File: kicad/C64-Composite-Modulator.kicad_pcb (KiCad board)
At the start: 2 copper layers, 63.5 x 60 mm, 56 parts, among them J1 Conn_01x04_Male, J2 Conn_01x04_Male, J3 Conn_01x04_Male, J4 Conn_01x04_Male, Q1 BC847B, Q2 BC847B, U1 78L05

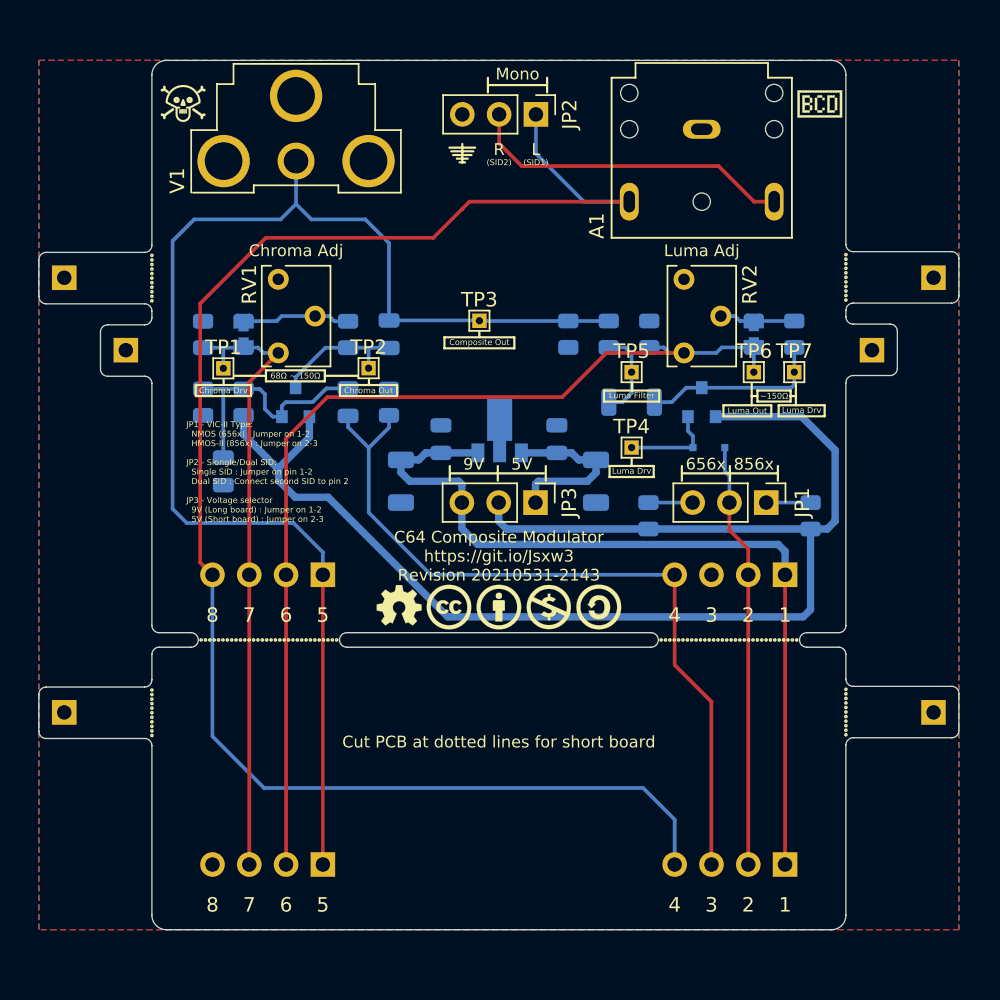
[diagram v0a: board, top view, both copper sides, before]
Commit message: Revision 20220130-1040
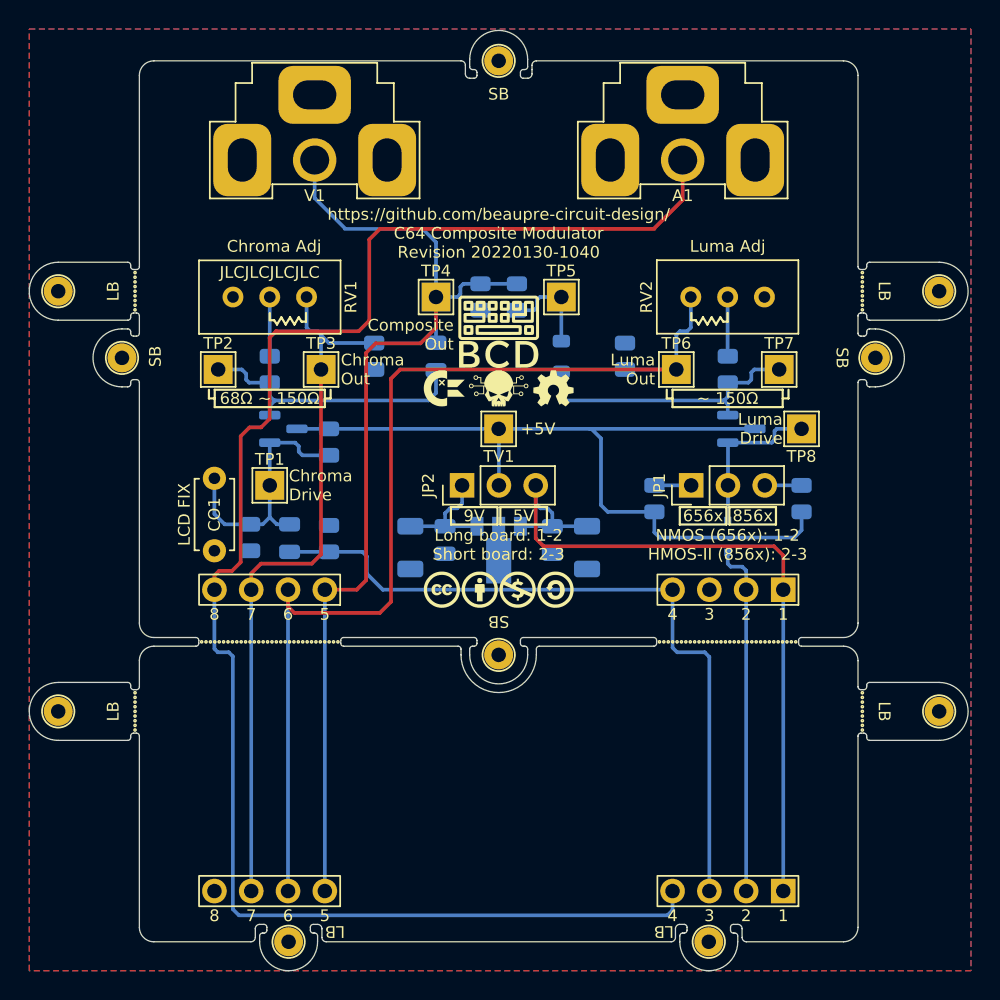
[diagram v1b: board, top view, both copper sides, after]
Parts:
- removed B1: RV1 Bypass, C64 Composite Modulator:J_0805_2012Metric
- removed B2: RV2 Bypass, C64 Composite Modulator:J_0805_2012Metric
- removed BCD1: BCD(DOT), BCD:BCD_LOGO_DOT-xxxsmall
- removed BY1: CC-BY, BCD:CC-BY-xxxsmall
- removed CC1: CC, BCD:CC-Logo-xxxsmall
- removed Danger1: Danger, BCD:Danger-xxxsmall
- removed J1, J2, J3, J4: Conn_01x04_Male, C64 Composite Modulator:mill-max-800-10-004-10-001000
- removed JP3: Jumper_3_Open, Connector_PinHeader_2.54mm:PinHeader_1x03_P2.54mm_Vertical
- removed LB1, LB2, LB3, LB4, SB1, SB2: Conn_01x01_Male, C64 Composite Modulator:mill-max-800-10-001-10-001000
- removed NC1: CC-NC, BCD:CC-NC-xxxsmall
- removed OSHW1: OSHW, BCD:OSHW-xxxsmall
- removed SA1: CC-SA, BCD:CC-SA-xxxsmall
- added CLB1: Modulator_Board_To_Long_Board, C64 Composite Modulator:Modulator to Long-Board support, F.Cu at (140.8, 105.4)
- added CSB1: Modulator_Board_To_Short_Board, C64 Composite Modulator:Modulator to Short-Board support, F.Cu at (140.8, 104.9)
- added G1: BCD_Logo, BeaupreCircuitDesign:BCD_Logo_5mm, F.Cu at (140.8, 93.7)
- added G2: ChickenLips, BeaupreCircuitDesign:ChickenLips_2.5mm, F.Cu at (137.0, 97.6)
- added G3: OpenSource_Hardware, BeaupreCircuitDesign:Open_Source_Hardware_2.5mm, F.Cu at (144.6, 97.6)
- added G4: Skull, BeaupreCircuitDesign:Skull_2.5mm, F.Cu at (140.8, 97.6)
- added G5: CreativeCommons, Creative_Common:CreativeCommons_2.5mm, F.Cu at (136.9, 111.5)
- added G6: CreativeCommons_Attribution, Creative_Common:CreativeCommons_Attribution_2.5mm, F.Cu at (139.5, 111.5)
- added G7: CreativeCommons_NonCommercial, Creative_Common:CreativeCommons_NonCommercial_2.5mm, F.Cu at (142.1, 111.5)
- added G8: CreativeCommons_ShareAlike, Creative_Common:CreativeCommons_ShareAlike_2.5mm, F.Cu at (144.7, 111.5)
- added TP8: TestPoint, TestPoint:TestPoint_THTPad_2.0x2.0mm_Drill1.0mm, F.Cu at (161.7, 100.4)
- added TV1: TestPoint, TestPoint:TestPoint_THTPad_2.0x2.0mm_Drill1.0mm, F.Cu at (140.8, 100.4)
- A1: value SJ1-3523N -> Conn_Coaxial; footprint C64 Composite Modulator:CUI_SJ1-3523N -> CUI_Devices:RCJ-013
- CO1: renamed from C7; footprint Capacitor_SMD:C_0805_2012Metric -> Capacitor_THT:C_Disc_D4.7mm_W2.5mm_P5.00mm; moved to F.Cu
- D1: value 1N4148 -> 1N4148WS
- L1: footprint Inductor_SMD:L_1206_3216Metric -> Inductor_SMD:L_0805_2012Metric
- Q1, Q2: value BC847B -> BC847C
- R1, R7: value 1K -> 1KΩ
- R10: value 75 -> 75Ω
- R11, R8, R9: value 150 -> 150Ω
- R2: value 3K3 -> 3K3Ω
- R3: value 5K6 -> 5K6Ω
- R4: value 68 -> 68Ω
- R5: value 220 -> 220Ω
- R6: value 470 -> 470Ω
- RV1: value 200 -> 1KΩ; footprint Potentiometer_THT:Potentiometer_Bourns_3266W_Vertical -> Potentiometer_THT:Potentiometer_Bourns_3296W_Vertical
- RV2: value 200 -> 500Ω; footprint Potentiometer_THT:Potentiometer_Bourns_3266W_Vertical -> Potentiometer_THT:Potentiometer_Bourns_3296W_Vertical
- TP1, TP2, TP3, TP4, TP5, TP6, TP7: footprint TestPoint:TestPoint_THTPad_1.0x1.0mm_Drill0.5mm -> TestPoint:TestPoint_THTPad_2.0x2.0mm_Drill1.0mm
- U1: value 78L05 -> 78L05G-AB3-R
- V1: footprint C64 Composite Modulator:CUI_RCJ-014 -> CUI_Devices:RCJ-014
- moved JP2 26.1 mm to (138.3, 104.3), turned to 90 degrees
- moved TP4 17.0 mm to (136.5, 91.3)
- moved C1 13.6 mm to (146.9, 108.6)
- moved C4 13.6 mm to (134.7, 108.6)
- moved R5 11.9 mm to (132.2, 95.4), turned to -90 degrees
- moved TP3 11.4 mm to (128.5, 96.3), turned to 180 degrees
- moved R6 10.8 mm to (151.5, 105.2), turned to -90 degrees
- moved R7 10.6 mm to (161.7, 105.2), turned to -90 degrees
- moved C3 10.4 mm to (137.1, 108.1), turned to -90 degrees
- moved TP2 10.4 mm to (121.4, 96.3), turned to 180 degrees
- moved C2 10.4 mm to (144.5, 108.1), turned to -90 degrees
- moved R1 10.3 mm to (129.1, 108.0), turned to -90 degrees
- moved C5 10.2 mm to (126.3, 108.0), turned to -90 degrees
- moved R3 9.89 mm to (123.6, 107.9)
- moved TP1 8.69 mm to (125.0, 104.3), turned to 180 degrees
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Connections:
- A1 pad 1: GND -> AudioIn
- A1 pad 2: AudioIn -> GND
- C5 pad 1: ChromaIn -> Net-(C5-Pad1)
- C5 pad 2: Net-(C5-Pad2) -> ChromaIn
- C6 pad 1: Net-(C6-Pad1) -> CompositeOut
- C6 pad 2: CompositeOut -> Net-(C6-Pad2)
- CO1 pad 1: Net-(C5-Pad2) -> Net-(C5-Pad1)
- JP1 pad 2: LumaIn -> Net-(D1-Pad2)
- JP2 pad 1: AudioIn -> Net-(C3-Pad1)
- JP2 pad 2: Net-(A1-Pad3) -> +5V
- JP2 pad 3: GND -> VCC
- Q1 pad 1: +5V -> Net-(C5-Pad1)
- Q1 pad 2: Net-(C5-Pad2) -> Net-(C6-Pad2)
- Q1 pad 3: Net-(C6-Pad1) -> +5V
- Q2 pad 1: +5V -> Net-(D1-Pad2)
- Q2 pad 2: Net-(D1-Pad2) -> Net-(L1-Pad2)
- Q2 pad 3: Net-(L1-Pad1) -> +5V
- R1 pad 1: ChromaIn -> GND
- R1 pad 2: GND -> ChromaIn
- R10 pad 2: Net-(L1-Pad1) -> Net-(L1-Pad2)
- R11 pad 1: LumaOut -> GND
- R11 pad 2: GND -> LumaOut
- R2 pad 2: Net-(C5-Pad2) -> Net-(C5-Pad1)
- R3 pad 1: Net-(C5-Pad2) -> Net-(C5-Pad1)
- R4 pad 2: Net-(C6-Pad1) -> Net-(C6-Pad2)
- R6 pad 1: +5V -> Net-(JP1-Pad1)
- R6 pad 2: Net-(JP1-Pad1) -> +5V
- R7 pad 1: +5V -> Net-(JP1-Pad3)
- R7 pad 2: Net-(JP1-Pad3) -> +5V
- R8 pad 2: Net-(L1-Pad2) -> Net-(L1-Pad1)
- R9 pad 1: GND -> CompositeOut
- R9 pad 2: CompositeOut -> GND
- RV1 pad 1: (no net) -> ChromaOut
- RV1 pad 3: ChromaOut -> unconnected-(RV1-Pad3)
- RV2 pad 1: (no net) -> LumaOut
- RV2 pad 3: LumaOut -> unconnected-(RV2-Pad3)
- TP1 pad 1: ChromaOut -> Net-(C5-Pad1)
- TP2 pad 1: Net-(C6-Pad1) -> Net-(C6-Pad2)
- TP3 pad 1: CompositeOut -> ChromaOut
- TP4 pad 1: Net-(D1-Pad2) -> CompositeOut
- TP5 pad 1: Net-(L1-Pad2) -> Net-(L1-Pad1)
- TP7 pad 1: Net-(L1-Pad1) -> Net-(L1-Pad2)
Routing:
- net +5V: track 95.4 -> 58.1 mm
- net Net-(A1-Pad3): track 22.7 -> 0.00 mm
- net Net-(C6-Pad2): track 0.00 -> 19.6 mm
- net CompositeOut: track 92.2 -> 72.7 mm
- net Net-(C5-Pad1): track 0.00 -> 18.2 mm
- net Net-(C5-Pad2): track 17.4 -> 0.00 mm
- net Net-(L1-Pad2): track 6.29 -> 19.7 mm
- net Net-(C6-Pad1): track 9.43 -> 0.00 mm
- net ChromaOut: track 42.9 -> 49.6 mm
- net VCC: track 58.5 -> 52.6 mm
- net Net-(L1-Pad1): track 12.7 -> 6.78 mm
- net LumaOut: track 68.6 -> 74.2 mm
- net LumaIn: track 29.5 -> 24.4 mm
- net Net-(D1-Pad2): track 6.51 -> 11.2 mm
- net Net-(C3-Pad1): track 12.0 -> 8.20 mm
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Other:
- board size 63.5 x 60 mm -> 64.8 x 64.9 mm
- net class Default removed
- net class Power removed
- board text added: "+5V"
- board text added: "68Ω ~ 150Ω"
- board text added: "Chroma Drive"
- board text added: "Cut PCB at dotted lines for C64C (Short) board"
- board text added: "JLCJLCJLCJLC"
- board text added: "LB"
- board text added: "LCD FIX"
- board text added: "Long board: 1-2 Short board: 2-3"
- board text added: "Luma Drive"
- board text added: "NMOS (656x): 1-2 HMOS-II (856x): 2-3"
- board text added: "SB"
- board text added: "https://github.com/beaupre-circuit-design/ C64 Composite Modulator Revision 20220130-1040"
- board text added: "~ 150Ω"
- board text removed: "(SID1)"
- board text removed: "(SID2)"
- board text removed: "1"
- board text removed: "2"
- board text removed: "3"
- board text removed: "4"
- board text removed: "5"
- board text removed: "6"
- board text removed: "68Ω ~~ 150Ω"
- board text removed: "7"
- board text removed: "8"
- board text removed: "C64 Composite Modulator https://git.io/Jsxw3 Revision 20210531-2143"
- board text removed: "Chroma Drv"
- board text removed: "Cut PCB at dotted lines for short board"
- board text removed: "JP1 - VIC-II Type: NMOS (656x) : Jumper on 1-2 HMOS-II (856x) : Jumper on 2-3 JP2 - Siongle/Dual SID: Single SID : Jumper on pin 1-2 Dual SID : Connect second SID to pin 2 JP3 - Voltage selector 9V (Long board) : Jumper on 1-2 5V (Short board) : Jumper on 2-3"
- board text removed: "L"
- board text removed: "Luma Drv"
- board text removed: "Luma Filter"
- board text removed: "Mono"
- board text removed: "R"
- board text removed: "~~150Ω"
